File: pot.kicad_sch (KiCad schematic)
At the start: 1 part

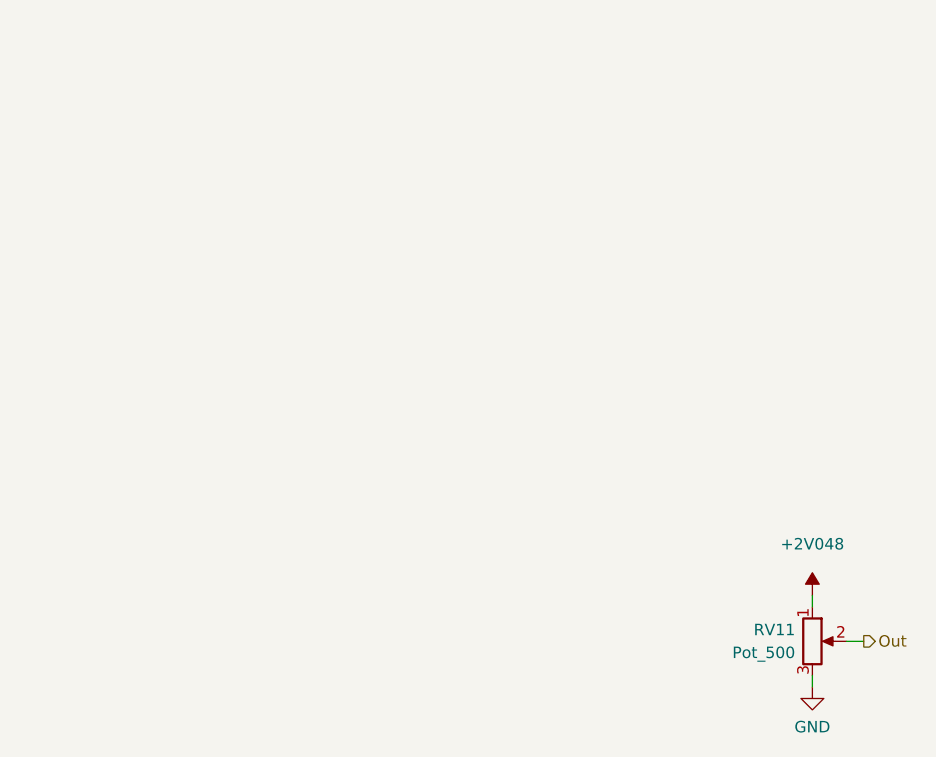
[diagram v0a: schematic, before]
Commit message: working on AD inputs
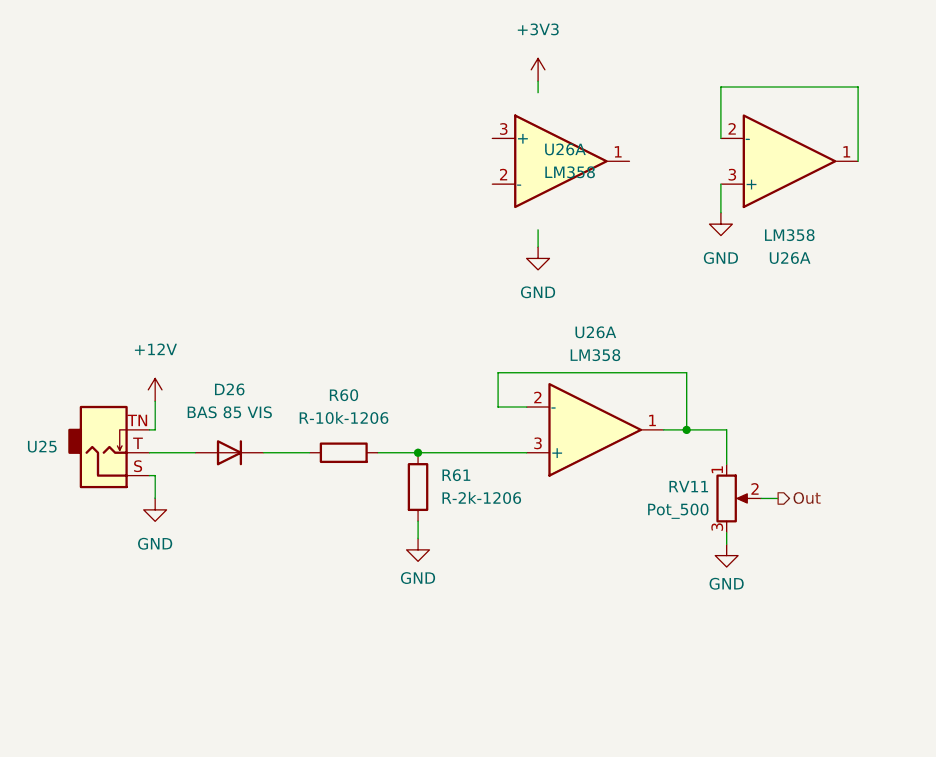
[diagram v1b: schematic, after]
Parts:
- added D26: BAS 85 VIS, Diode_SMD:D_MiniMELF, symbol eurorack:BAS 85 VIS
- added R60: R-10k-1206, Resistor_SMD:R_1206_3216Metric_Pad1.30x1.75mm_HandSolder, symbol eurorack:R-10k-1206
- added R61: R-2k-1206, Resistor_SMD:R_1206_3216Metric_Pad1.30x1.75mm_HandSolder, symbol eurorack:R-2k-1206
- added U25: LUM-1502-03_3.5mm_mono_vertical_jack, eurorack:LUM 1502-03, symbol eurorack:LUM-1502-03_3.5mm_mono_vertical_jack
- added U26 (x3): LM358, Package_SO:SO-8_3.9x4.9mm_P1.27mm, symbol eurorack:LM358
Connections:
- net GND: now also R61.2, U25.S, U26.3 (+)
- net 1V25: no longer names the net of RV11.1
- net 1V25: now also U26.1, U26.2 (-)
- new net: D26.1 (A), U25.T
- new net: D26.2 (K), R60.1
- new net: R60.2, R61.1, U26.3 (+)
- new net: U26.1, U26.2 (-)
- new net +12V: U25.TN
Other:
- moved on the sheet: RV11
